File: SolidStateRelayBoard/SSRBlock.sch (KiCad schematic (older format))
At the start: 8 parts, among them Q201 MMBT2222ALT1G, U201 SSR

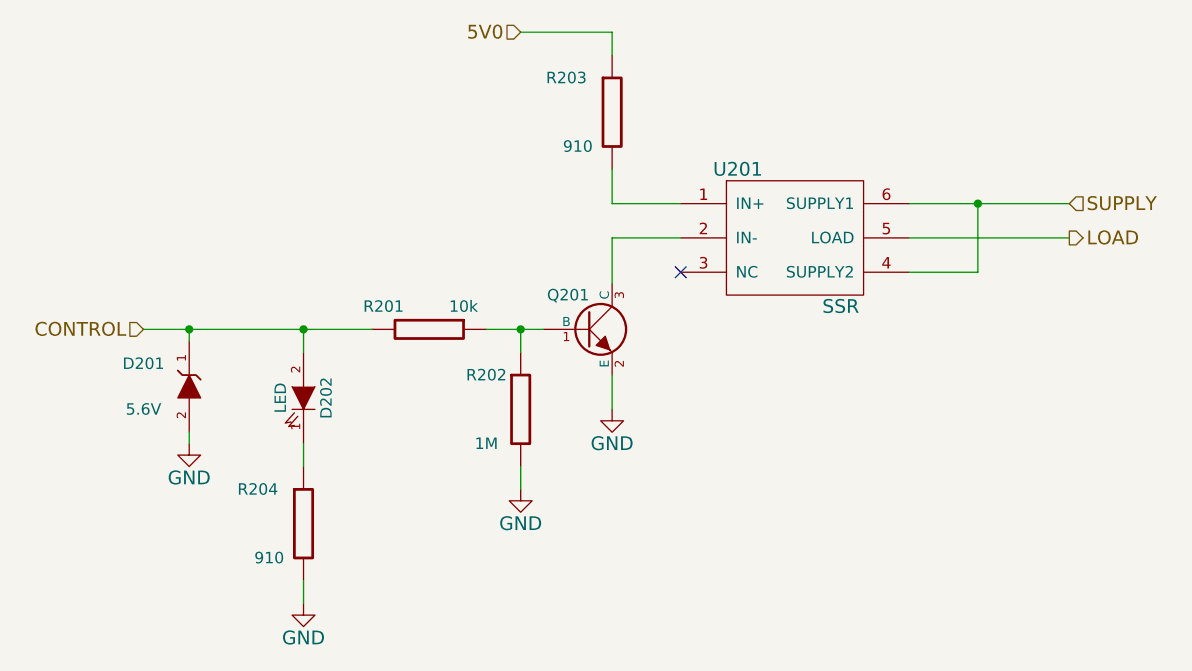
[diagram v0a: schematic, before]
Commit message: SSR Board
Misc small changes
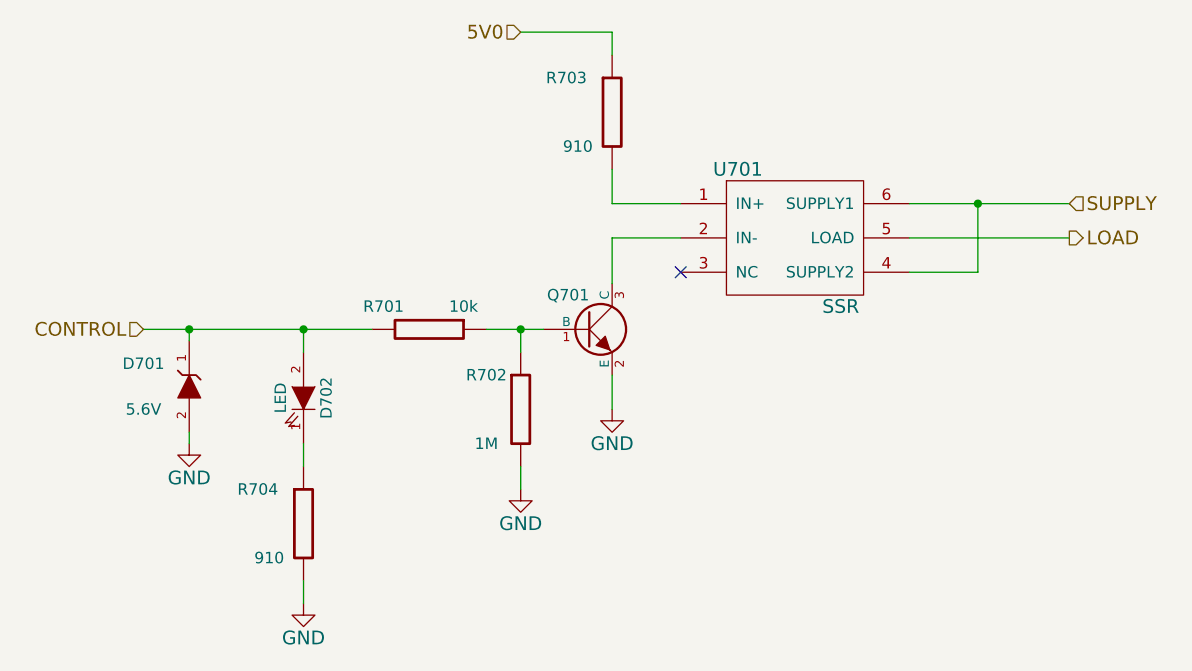
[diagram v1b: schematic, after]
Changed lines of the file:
@@
 $Descr A4 11693 8268
 encoding utf-8
-Sheet 2 14
+Sheet 7 14
 Title ""
 Date ""
@@
 AR Path="/586B7988/586B33BB" Ref="Q1601"  Part="1"
 AR Path="/586B7996/586B33BB" Ref="Q1701"  Part="1"
-F 0 "Q201" H 5100 3400 50  0000 R CNN
+F 0 "Q701" H 5100 3400 50  0000 R CNN
 F 1 "MMBT2222ALT1G" H 5100 3400 50  0001 R CNN
 F 2 "TO_SOT_Packages_SMD:SOT-23_Handsoldering" H 5100 3250 60  0001 C CNN
@@
 AR Path="/586B7988/586B33E9" Ref="R1603"  Part="1"
 AR Path="/586B7996/586B33E9" Ref="R1703"  Part="1"
-F 0 "R203" H 5000 2450 50  0000 C CNN
+F 0 "R703" H 5000 2450 50  0000 C CNN
 F 1 "910" H 5050 2150 50  0000 C CNN
 F 2 "Resistors_SMD:R_1206_HandSoldering" V 5130 2300 30  0001 C CNN
@@
 AR Path="/586B7988/586B3431" Ref="R1601"  Part="1"
 AR Path="/586B7996/586B3431" Ref="R1701"  Part="1"
-F 0 "R201" V 4300 3050 50  0000 C CNN
+F 0 "R701" V 4300 3050 50  0000 C CNN
 F 1 "10k" V 4300 3400 50  0000 C CNN
 F 2 "Resistors_SMD:R_1206_HandSoldering" V 4330 3250 30  0001 C CNN
@@
 AR Path="/586B7988/586B354B" Ref="#PWR091"  Part="1"
 AR Path="/586B7996/586B354B" Ref="#PWR095"  Part="1"
-F 0 "#PWR084" H 5200 3350 60  0001 C CNN
+F 0 "#PWR056" H 5200 3350 60  0001 C CNN
 F 1 "GND" H 5200 3450 60  0000 C CNN
 F 2 "" H 5200 3600 60  0000 C CNN
@@
 AR Path="/586B7988/586B3681" Ref="D1601"  Part="1"
 AR Path="/586B7996/586B3681" Ref="D1701"  Part="1"
-F 0 "D201" V 3450 3700 50  0000 C CNN
+F 0 "D701" V 3450 3700 50  0000 C CNN
 F 1 "5.6V" V 3250 3700 50  0000 C CNN
 F 2 "hyperCustom:SOD-123" H 3350 3500 60  0001 C CNN
@@
 AR Path="/586B7988/586B36D9" Ref="#PWR092"  Part="1"
 AR Path="/586B7996/586B36D9" Ref="#PWR096"  Part="1"
-F 0 "#PWR085" H 3350 3500 60  0001 C CNN
+F 0 "#PWR057" H 3350 3500 60  0001 C CNN
 F 1 "GND" H 3350 3600 60  0000 C CNN
 F 2 "" H 3350 3750 60  0000 C CNN
@@
 AR Path="/586B7988/586B39A4" Ref="R1602"  Part="1"
 AR Path="/586B7996/586B39A4" Ref="R1702"  Part="1"
-F 0 "R202" H 4650 3750 50  0000 C CNN
+F 0 "R702" H 4650 3750 50  0000 C CNN
 F 1 "1M" H 4650 3450 50  0000 C CNN
 F 2 "Resistors_SMD:R_1206_HandSoldering" V 4730 3600 30  0001 C CNN
@@
 AR Path="/586B7988/586B3A19" Ref="#PWR093"  Part="1"
 AR Path="/586B7996/586B3A19" Ref="#PWR097"  Part="1"
-F 0 "#PWR086" H 4800 3700 60  0001 C CNN
+F 0 "#PWR058" H 4800 3700 60  0001 C CNN
 F 1 "GND" H 4800 3800 60  0000 C CNN
 F 2 "" H 4800 3950 60  0000 C CNN
@@
 AR Path="/586B7988/586D88E1" Ref="U1601"  Part="1"
 AR Path="/586B7996/586D88E1" Ref="U1701"  Part="1"
-F 0 "U201" H 5750 3150 60  0000 C CNN
+F 0 "U701" H 5750 3150 60  0000 C CNN
 F 1 "SSR" H 6200 2550 60  0000 C CNN
 F 2 "hyperCustom:VISHAY_6SMD_OPTOCOUPLER" H 6000 2850 60  0001 C CNN
@@
 AR Path="/586B7996/586E6B18" Ref="D1702"  Part="1"
 AR Path="/586E6B18" Ref="D202"  Part="1"
-F 0 "D202" H 3850 3650 50  0000 C CNN
+F 0 "D702" H 3850 3650 50  0000 C CNN
 F 1 "LED" H 3850 3450 50  0000 C CNN
 F 2 "hyperCustom:SOD-123" H 3850 3550 60  0001 C CNN
@@
 AR Path="/586B7988/586E6B5D" Ref="R1604"  Part="1"
 AR Path="/586B7996/586E6B5D" Ref="R1704"  Part="1"
-F 0 "R204" H 3650 4250 50  0000 C CNN
+F 0 "R704" H 3650 4250 50  0000 C CNN
 F 1 "910" H 3700 3950 50  0000 C CNN
 F 2 "Resistors_SMD:R_1206_HandSoldering" V 3780 4100 30  0001 C CNN
@@
 AR Path="/586B7988/586E6C2B" Ref="#PWR094"  Part="1"
 AR Path="/586B7996/586E6C2B" Ref="#PWR098"  Part="1"
-F 0 "#PWR087" H 3850 4200 60  0001 C CNN
+F 0 "#PWR059" H 3850 4200 60  0001 C CNN
 F 1 "GND" H 3850 4300 60  0000 C CNN
 F 2 "" H 3850 4450 60  0000 C CNN
